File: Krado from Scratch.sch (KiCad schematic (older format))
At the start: 157 parts, among them SW1 SW_Push, U1 ATmega32U4-AU, Y1 16MHz

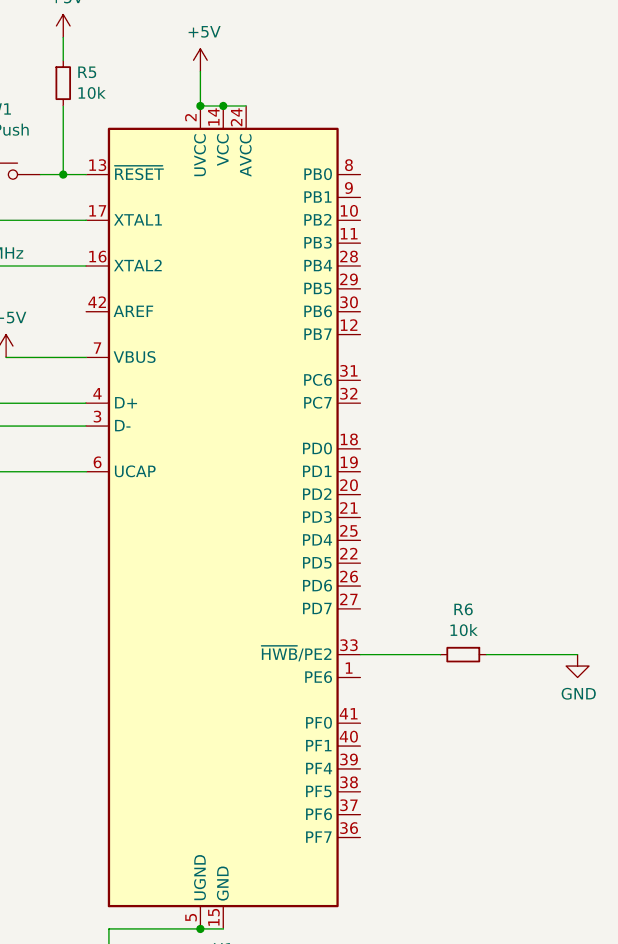
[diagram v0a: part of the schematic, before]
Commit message: PCB Mapped
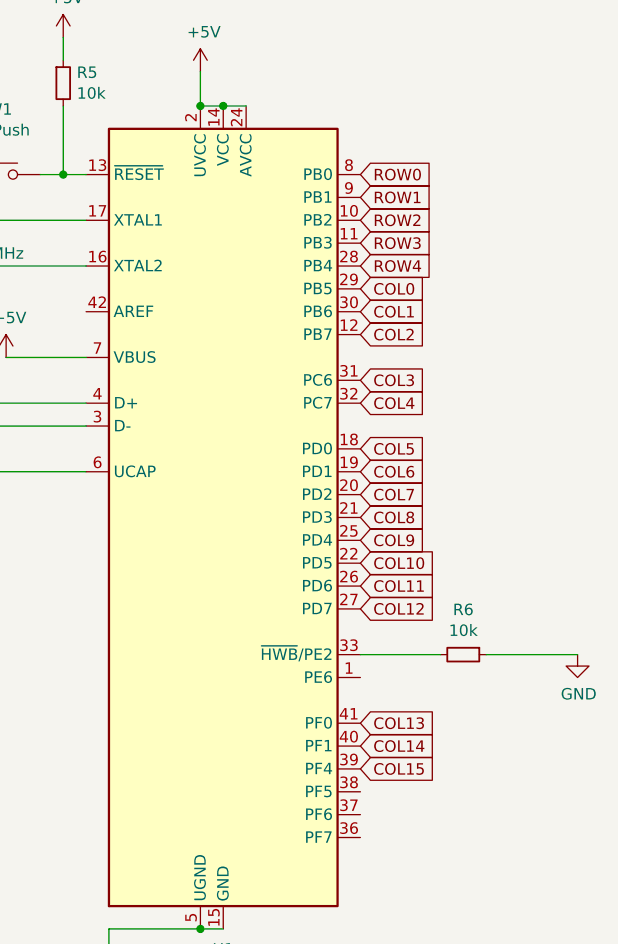
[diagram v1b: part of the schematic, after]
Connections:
- net COL0: now also U1.29 (PB5)
- net COL1: now also U1.30 (PB6)
- net COL10: now also U1.22 (PD5)
- net COL11: now also U1.26 (PD6)
- net COL12: now also U1.27 (PD7)
- net COL13: now also U1.41 (PF0)
- net COL14: now also U1.40 (PF1)
- net COL15: now also U1.39 (PF4)
- net COL2: now also U1.12 (PB7)
- net COL3: now also U1.31 (PC6)
- net COL4: now also U1.32 (PC7)
- net COL5: now also U1.18 (PD0)
- net COL6: now also U1.19 (PD1)
- net COL7: now also U1.20 (PD2)
- net COL8: now also U1.21 (PD3)
- net COL9: now also U1.25 (PD4)
- net ROW0: now also U1.8 (PB0)
- net ROW1: now also U1.9 (PB1)
- net ROW2: now also U1.10 (PB2)
- net ROW3: now also U1.11 (PB3)
- net ROW4: now also U1.28 (PB4)
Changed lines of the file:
@@
 Wire Wire Line
 	17750 7650 17750 7550
+Text GLabel 21050 7450 2    50   Input ~ 0
+ROW0
+Text GLabel 21050 7550 2    50   Input ~ 0
+ROW1
+Text GLabel 21050 7650 2    50   Input ~ 0
+ROW2
+Text GLabel 21050 7750 2    50   Input ~ 0
+ROW3
+Text GLabel 21050 7850 2    50   Input ~ 0
+ROW4
+Text GLabel 21050 7950 2    50   Input ~ 0
+COL0
+Text GLabel 21050 8050 2    50   Input ~ 0
+COL1
+Text GLabel 21050 8150 2    50   Input ~ 0
+COL2
+Text GLabel 21050 8350 2    50   Input ~ 0
+COL3
+Text GLabel 21050 8450 2    50   Input ~ 0
+COL4
+Text GLabel 21050 8650 2    50   Input ~ 0
+COL5
+Text GLabel 21050 8750 2    50   Input ~ 0
+COL6
+Text GLabel 21050 8850 2    50   Input ~ 0
+COL7
+Text GLabel 21050 8950 2    50   Input ~ 0
+COL8
+Text GLabel 21050 9050 2    50   Input ~ 0
+COL9
+Text GLabel 21050 9150 2    50   Input ~ 0
+COL10
+Text GLabel 21050 9250 2    50   Input ~ 0
+COL11
+Text GLabel 21050 9350 2    50   Input ~ 0
+COL12
+Text GLabel 21050 9850 2    50   Input ~ 0
+COL13
+Text GLabel 21050 9950 2    50   Input ~ 0
+COL14
+Text GLabel 21050 10050 2    50   Input ~ 0
+COL15
 $EndSCHEMATC
